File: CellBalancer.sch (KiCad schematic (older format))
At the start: 12 parts, among them IC2 MAX923, Q2 IRF7455PBF

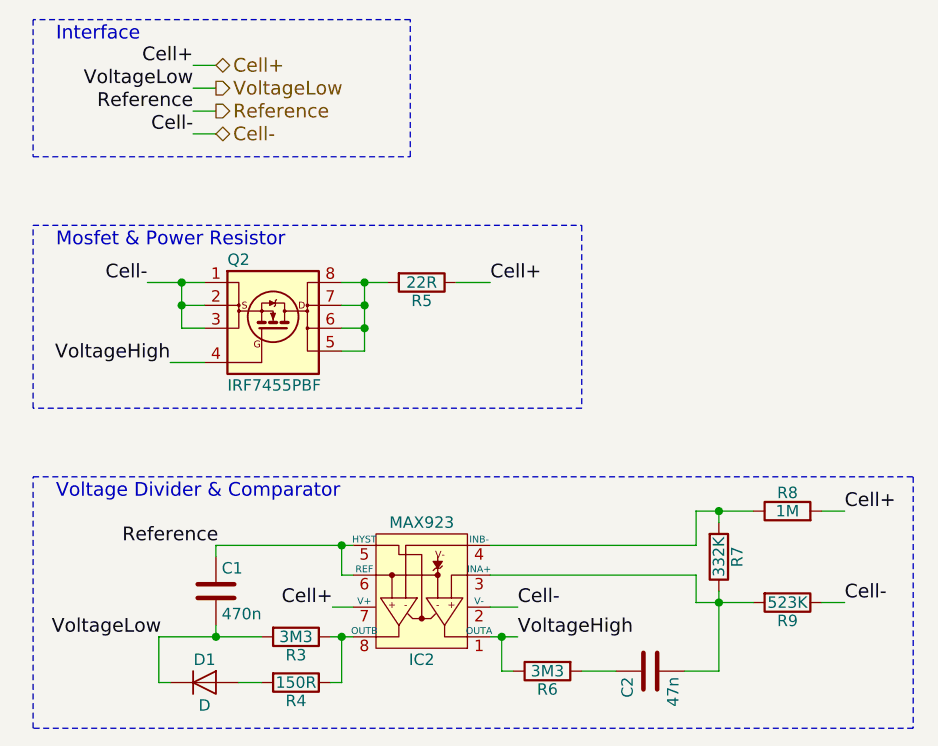
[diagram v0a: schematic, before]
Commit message: layout finalized
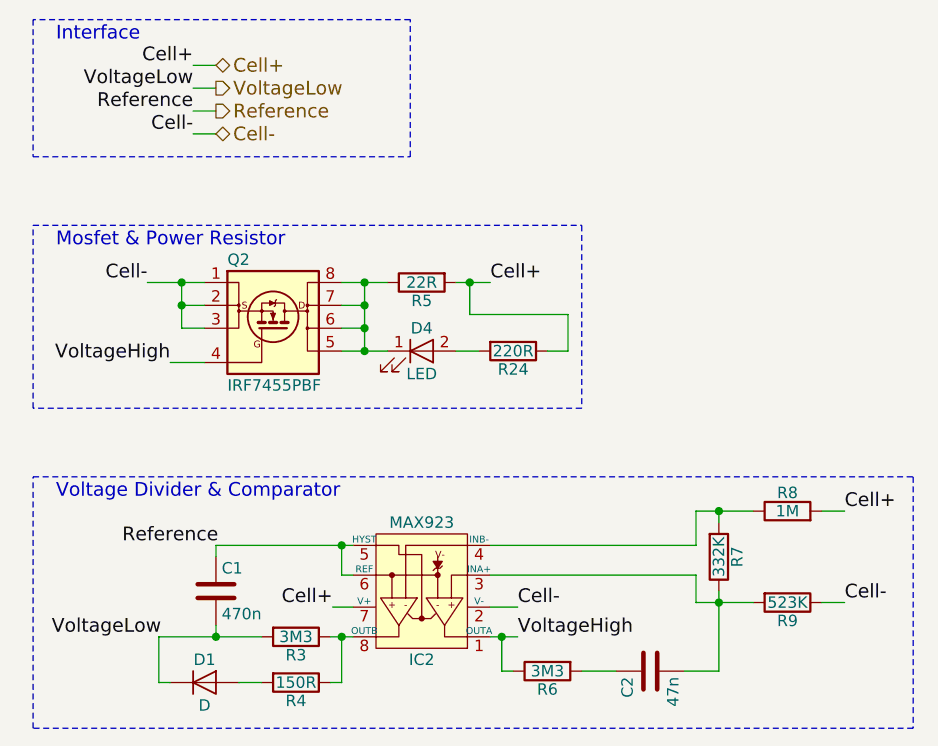
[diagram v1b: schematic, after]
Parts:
- added D4: LED, LEDs:LED_0805, symbol LED
- added R24: 220R, Resistors_SMD:R_0805, symbol R
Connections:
- net Cell+: now also R5.2, R24.1; no longer R5.1
- net at Q2.5 (D), Q2.6 (D), Q2.7 (D)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: now also R5.1, D4.1 (K); no longer R5.2
- new net: D4.2 (A), R24.2
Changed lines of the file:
@@
 F 3 "" H 2800 1950 50  0001 C CNN
 	1    2800 1950
-	0    1    1    0
+	0    -1   1    0
 $EndComp
 $Comp
@@
 	2550 1950 2550 2250
 Wire Wire Line
-	2550 2250 2450 2250
+	2450 2250 2650 2250
 Connection ~ 2550 1950
 Wire Wire Line
@@
 Text Notes 1200 2900 0    60   ~ 0
 Voltage Divider & Comparator
+$Comp
+L R R24
+U 1 1 58CFD09E
+P 3200 2250
+AR Path="/58CDDC72/58CFD09E" Ref="R24"  Part="1"
+AR Path="/58CDE720/58CFD09E" Ref="R25"  Part="1"
+AR Path="/58CDEEA6/58CFD09E" Ref="R26"  Part="1"
+F 0 "R24" V 3280 2250 50  0000 C CNN
+F 1 "220R" V 3200 2250 50  0000 C CNN
+F 2 "Resistors_SMD:R_0805" V 3130 2250 50  0001 C CNN
+F 3 "" H 3200 2250 50  0001 C CNN
+	1    3200 2250
+	0    1    1    0
+$EndComp
+$Comp
+L LED D4
+U 1 1 58CFD291
+P 2800 2250
+AR Path="/58CDDC72/58CFD291" Ref="D4"  Part="1"
+AR Path="/58CDE720/58CFD291" Ref="D5"  Part="1"
+AR Path="/58CDEEA6/58CFD291" Ref="D6"  Part="1"
+F 0 "D4" H 2800 2350 50  0000 C CNN
+F 1 "LED" H 2800 2150 50  0000 C CNN
+F 2 "LEDs:LED_0805" H 2800 2250 50  0001 C CNN
+F 3 "" H 2800 2250 50  0001 C CNN
+	1    2800 2250
+	1    0    0    -1
+$EndComp
+Connection ~ 2550 2250
+Wire Wire Line
+	2950 2250 3050 2250
+Wire Wire Line
+	3010 1950 3010 2090
+Wire Wire Line
+	3010 2090 3440 2090
+Wire Wire Line
+	3440 2090 3440 2250
+Wire Wire Line
+	3440 2250 3350 2250
+Connection ~ 3010 1950
 $EndSCHEMATC
